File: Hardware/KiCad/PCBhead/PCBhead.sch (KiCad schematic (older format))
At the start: 10 parts, among them IC2 OPT3002DNPT, J1 LEDazul, J2 LEDambar, J4 Vin

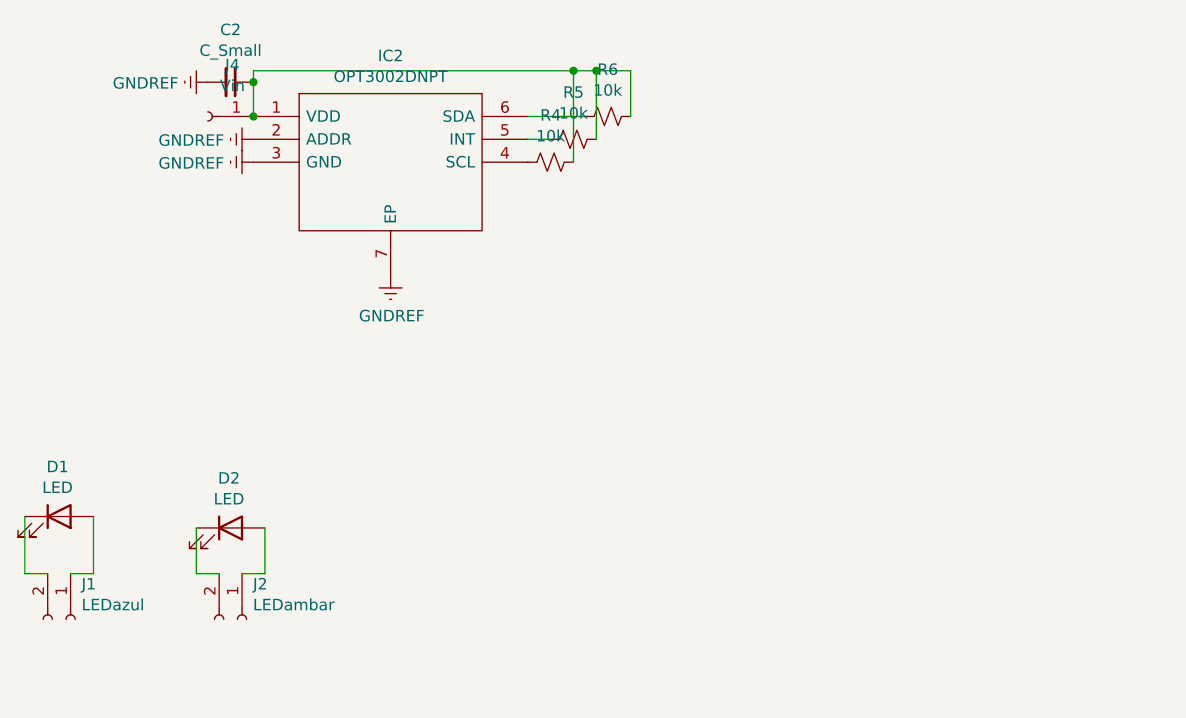
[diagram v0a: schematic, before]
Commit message: head update
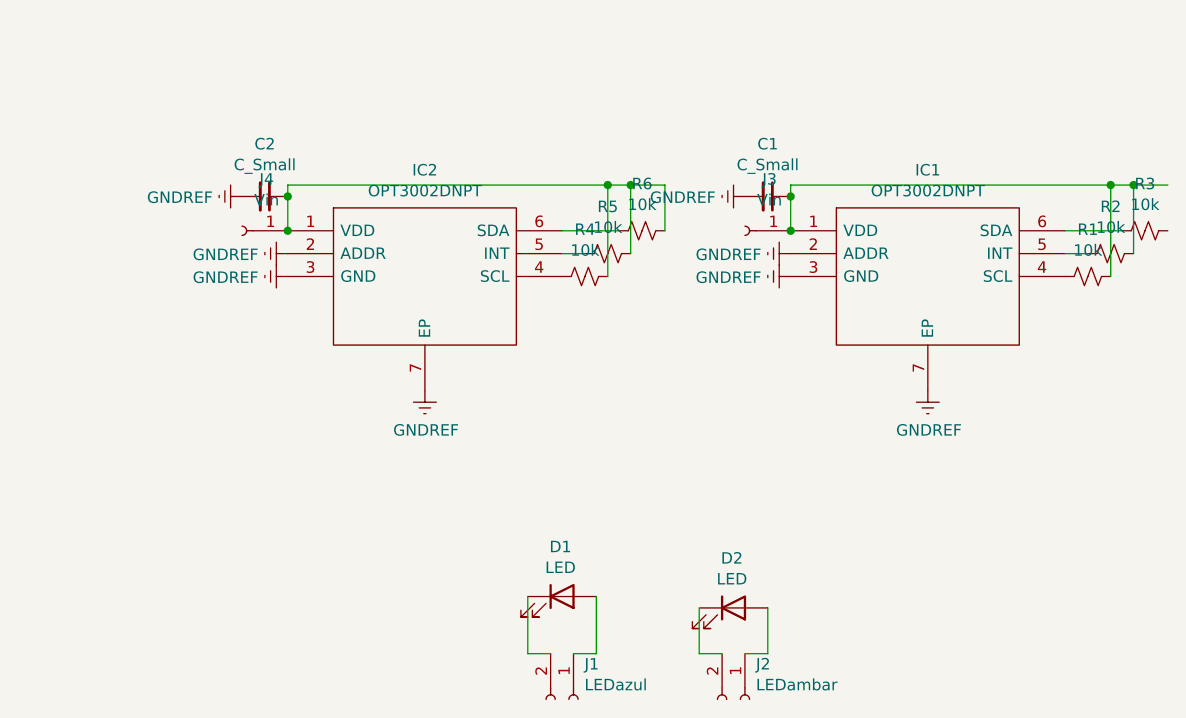
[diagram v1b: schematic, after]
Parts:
- added C1: C_Small, Capacitor_SMD:C_0805_2012Metric, symbol Device:C_Small
- added IC1: OPT3002DNPT, OPT3002DNPT:SON65P200X200X65-7N-D, symbol OPT3002DNPT:OPT3002DNPT
- added J3: Vin, Connector_PinSocket_2.54mm:PinSocket_1x01_P2.54mm_Horizontal, symbol Connector:Conn_01x01_Female
- added R1, R2, R3: 10k, Resistor_SMD:R_0805_2012Metric, symbol Device:R_Small_US
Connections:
- wire segments 18 -> 27
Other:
- moved on the sheet: C2, D1, D2, IC2, J1, J2, J4, R4, R5, R6
